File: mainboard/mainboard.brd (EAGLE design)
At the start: 93.7 x 52.1 mm, 23 parts, among them U1 DWM1000, U2 ESP8266

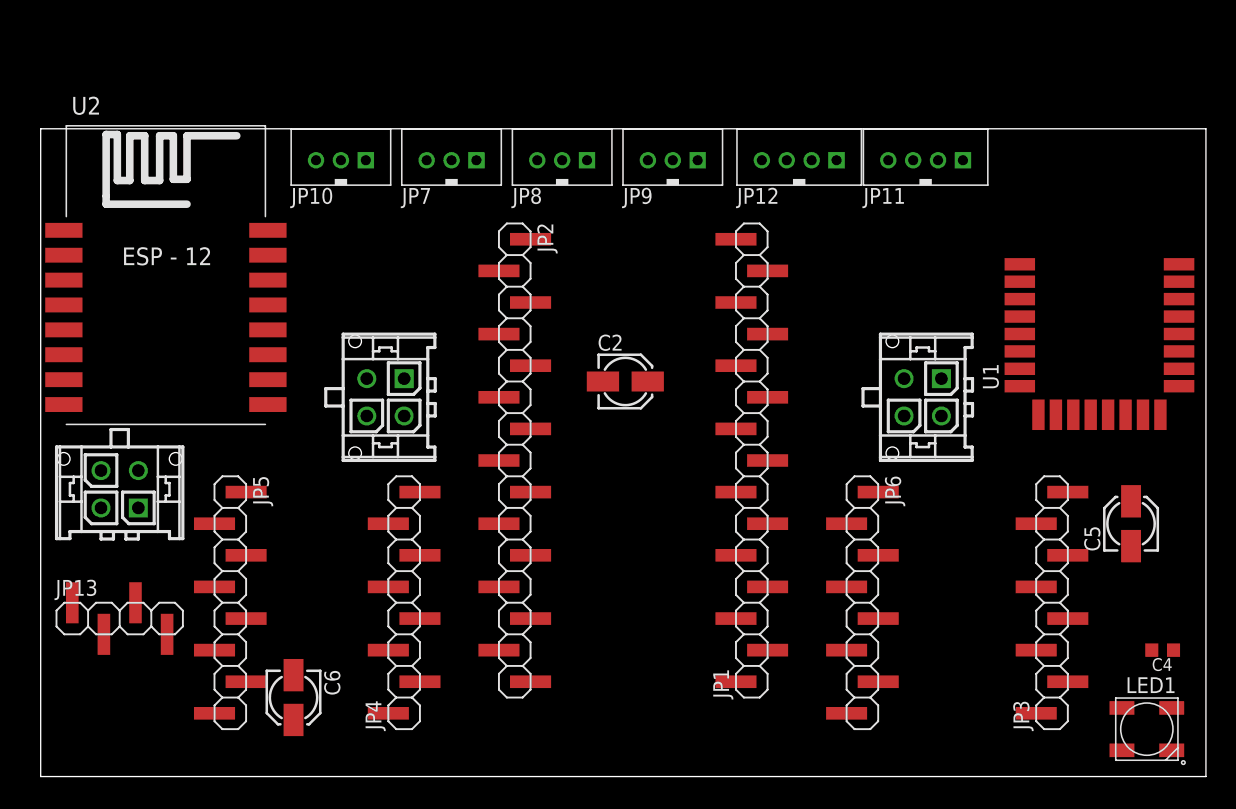
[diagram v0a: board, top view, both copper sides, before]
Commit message: boardf
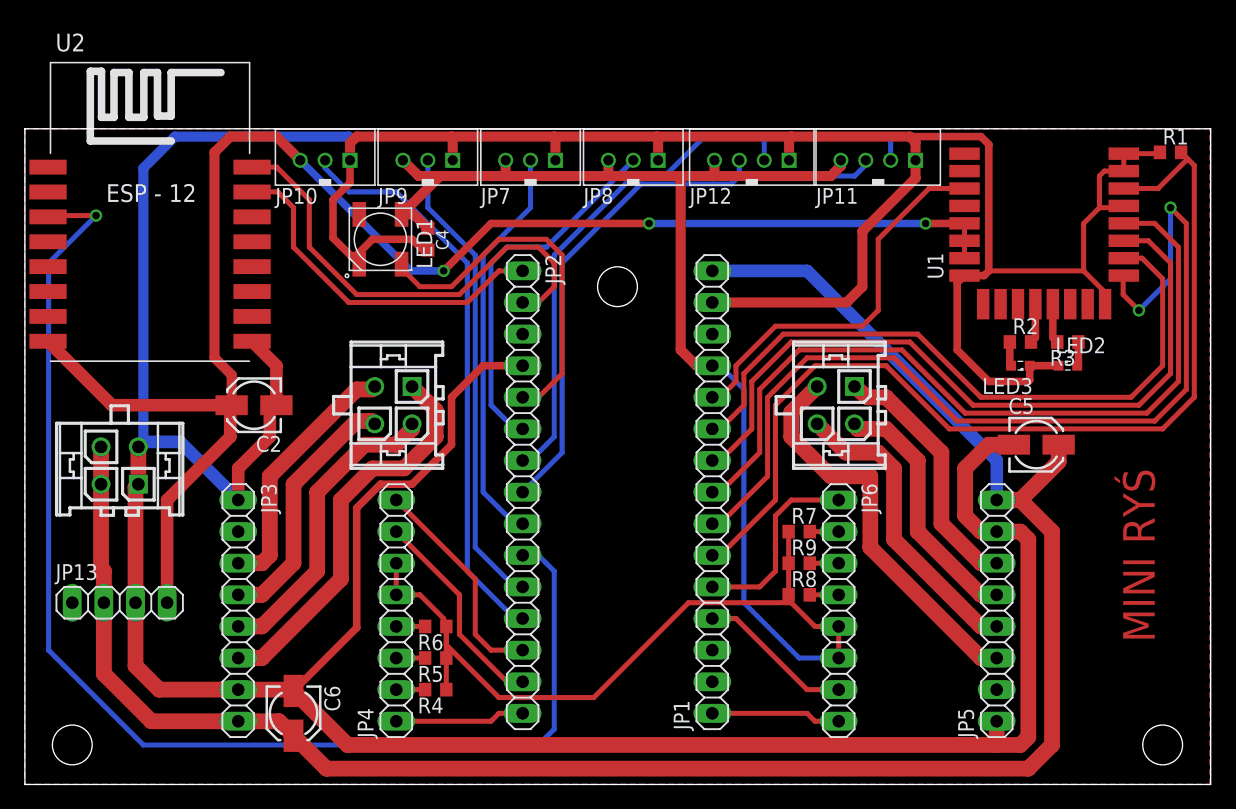
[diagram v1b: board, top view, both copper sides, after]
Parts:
- added LED2, LED3: (no value), led:SML0603
- added R1: 10k, rcl:R0603
- added R2, R3: 330R, rcl:R0603
- added R4, R5, R6, R7, R8, R9: (no value), rcl:R0603
- JP1, JP2: device pinhead-2:1X15SMD -> pinhead:1X15
- JP13: device pinhead-2:1X04SMD -> pinhead:1X04
- JP3, JP4, JP5, JP6: device pinhead-2:1X08SMD -> pinhead:1X08
- moved LED1 73.1 mm to (27.3, 43.2), turned to 270 degrees
- moved C4 67.7 mm to (31.1, 43.2), turned to 270 degrees
- moved JP3 65.8 mm to (15.9, 13.3), turned to 270 degrees
- moved JP5 62.1 mm to (76.8, 13.3), turned to 90 degrees
- moved X1 42.5 mm to (29.8, 29.8)
- moved X2 36.2 mm to (65.4, 29.8)
- moved C2 29.9 mm to (17.1, 29.8), turned to 180 degrees
- moved JP9 19.7 mm to (31.1, 49.5)
- moved JP2 19.1 mm to (38.7, 22.9)
- moved JP1 14.3 mm to (54.0, 22.9)
- moved U1 9.94 mm to (80.6, 48.3)
- moved C5 9.92 mm to (80.0, 26.7), turned to 0 degrees
- moved JP6 8.47 mm to (64.1, 13.3)
- moved JP4 7.01 mm to (28.6, 13.3)
- moved JP7 6.35 mm to (39.4, 49.5)
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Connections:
- removed net 5V: JP1.12
- removed net M0L: JP6.2
- removed net M0R: JP4.2
- removed net M1L: JP6.3
- removed net M1R: JP4.3
- removed net M2L: JP6.4
- removed net M2R: JP4.4
- removed net N$1 (its old number): JP9.1
- removed net N$13 (its old number): JP7.2
- removed net N$25: U1.3
- removed net N$26: JP10.1
- removed net N$27: JP10.2
- removed net P1: JP2.10
- removed net P2: JP2.11
- removed net P3: JP2.12
- removed net PA12: JP2.5
- removed net PA2: JP1.11
- removed net PA3: JP1.6
- removed net VDDAON: U1.5
- removed net VIN: JP1.15
- new net DWMRES: JP1.11, U1.3
- new net ESPEN: JP2.10, U2.CH_PD
- new net IRQ: JP1.6, R1.2, U1.22
- new net N$11: JP6.4, R8.2
- new net N$4: JP4.2, R4.2
- new net N$5: LED2.A, R3.1
- new net N$6: LED3.A, R2.1
- new net N$8: JP4.4, R6.2
- new net N$9: JP6.2, R7.2
- new net PWM1: JP10.2, JP2.12
- new net PWM2: JP2.11, JP9.2
- net +12V: now also JP1.15
- net +3V3: now also U1.5; no longer JP9.3
- net +5V: now also JP1.12, JP9.3, R4.1, R5.1, R6.1, R7.1, R8.1, R9.1
- net CSN: now also U1.17
- net GND: now also JP10.1, JP9.1, LED2.C, LED3.C, R1.1
- net LED1: now also JP2.5
- net N$10: now also JP6.3, R9.2; no longer JP8.2
- net N$2: now also R3.2, U1.13; no longer U2.CH_PD
- net N$3: now also R2.2, U1.12; no longer JP9.2
- net N$7: now also JP4.3, R5.2; no longer U1.17
- net PB0: now also JP8.2
- net PB1: now also JP7.2
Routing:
- net GND: track 0.00 -> 389.4 mm
- net +12V: track 0.00 -> 159.2 mm
- net +5V: track 0.00 -> 154.4 mm
- net +3V3: track 0.00 -> 125.4 mm, vias 0 -> 3
- net ESPEN: track 0.00 -> 100.5 mm, vias 0 -> 1
- net IRQ: track 0.00 -> 78.9 mm
- net CSN: track 0.00 -> 78.3 mm, vias 0 -> 2
- net SCK: track 0.00 -> 64.3 mm
- net MISO: track 0.00 -> 59.6 mm
- net MOSI: track 0.00 -> 54.8 mm
- net SDA: track 0.00 -> 52.6 mm
- net SCL: track 0.00 -> 49.0 mm
- net PWM1: track 0.00 -> 46.0 mm
- net RX: track 0.00 -> 37.8 mm
- net PWM2: track 0.00 -> 37.8 mm
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- added copper zone on layer 1, net GND
- added copper zone on layer 16, net GND
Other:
- board size 93.7 x 52.1 mm -> 95.3 x 52.7 mm
- board text added: "MINI RYŚ"
